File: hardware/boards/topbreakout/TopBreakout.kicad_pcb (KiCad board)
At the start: 2 copper layers, 75.6 x 73 mm, 46 parts, among them J1 WURTH_ELECTRONICS_61400413321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, J2 MOLEX_52892-3033MOLEX_52892-3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, J3 USB-A-S-X-X-VT, U1 ANALOG_DEVICES_AD7606BSTZANAL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, U3 ANALOG_DEVICES_AD5754BREZANAL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, U5 MICROCHIP_MCP1700T-2502E-TTMI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

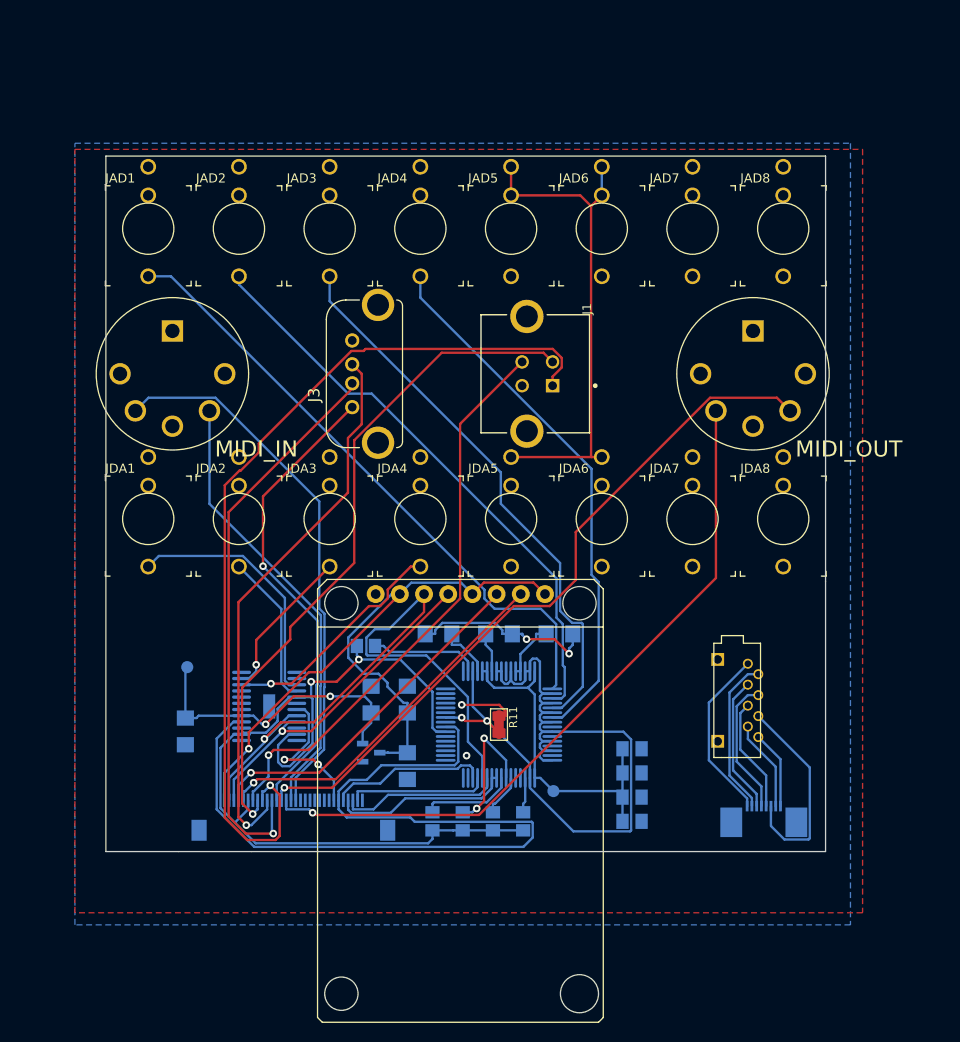
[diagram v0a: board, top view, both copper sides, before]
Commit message: cleanup
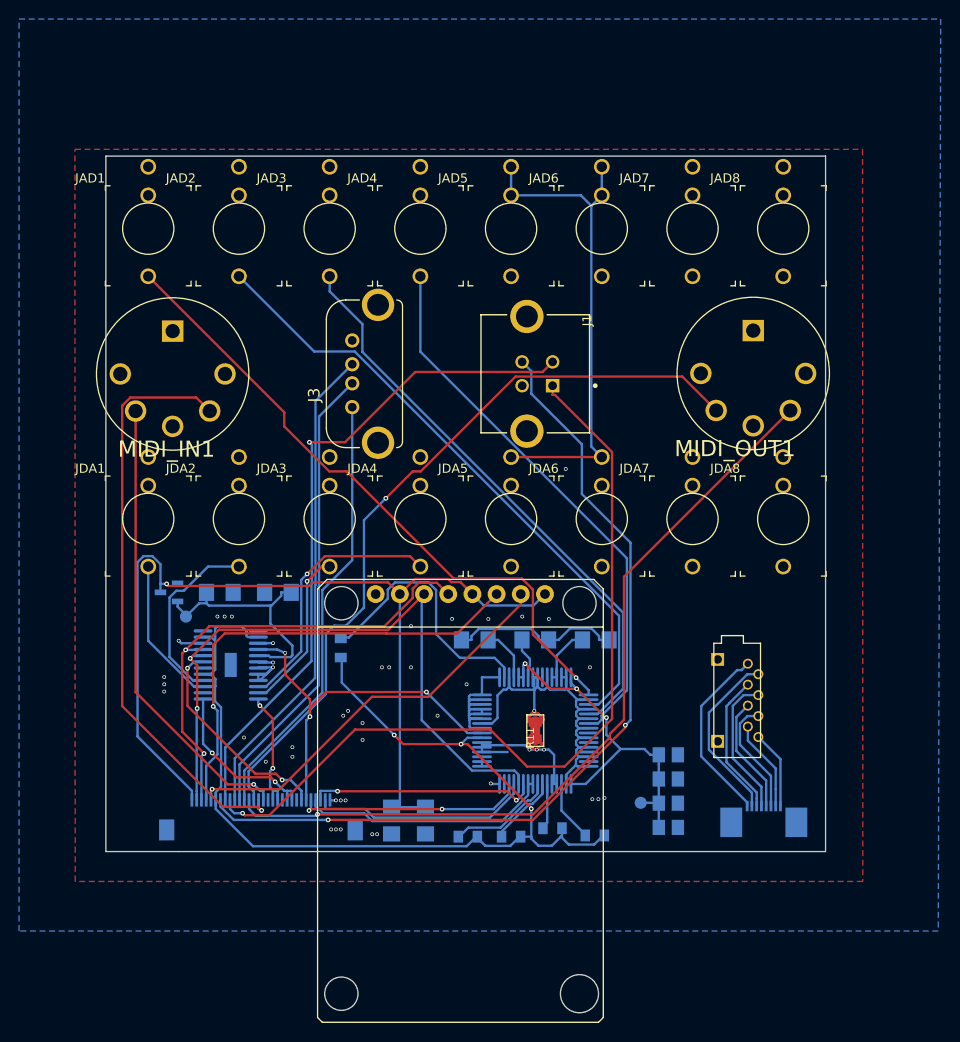
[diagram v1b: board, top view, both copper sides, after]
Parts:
- removed MIDI_IN, MIDI_OUT: OG-MIDI_MAB5SHCUI-SD-50BV, OG-MIDI_SD-50BV
- added MIDI_IN1: OG-MIDI_MAB5SHCUI-SD-50BV, topbreakout:OG-MIDI_SD-50BV, F.Cu at (117.7, 91.4)
- added MIDI_OUT1: OG-MIDI_MAB5SHCUI-SD-50BV, topbreakout:OG-MIDI_SD-50BV, F.Cu at (178.7, 91.3)
- C1, C2, C3, C4: footprint C0805K -> topbreakout:C0805K
- C10, C11, C6, C9: footprint C1206 -> topbreakout:C1206
- C5, C7, C8: footprint 1206 -> topbreakout:1206
- J1: footprint WURTH_ELECTRONICS_61400413321_0 -> topbreakout:WURTH_ELECTRONICS_61400413321_0
- J2: value MOLEX_52892-3033MOLEX_52892-3033_0_0 -> MOLEX_52892-3033; footprint MOLEX_52892-3033_0 -> topbreakout:MOLEX_52892-3033_0
- J3: footprint USB-A-S-X-X-VT -> topbreakout:USB-A-S-X-X-VT
- J4: value (none) -> ST7735_1.4; footprint ST7735 -> topbreakout:ST7735
- JAD1, JAD2, JAD3, JAD4, JAD5, JAD6, JAD7, JAD8, JDA1, JDA2, JDA3, JDA4, JDA5, JDA6, JDA7, JDA8: footprint WQP-PJ301M-12_JACK -> topbreakout:WQP-PJ301M-12_JACK
- R10, R4, R7, R8, R9: footprint R0805 -> Capacitors_SMD:C_0805
- R11: footprint R0805 -> topbreakout:R0805
- TP1, TP3: footprint PAD.03X.05 -> topbreakout:PAD.03X.05
- U$1: footprint YAMAICHI_MICROSD_VERTICAL -> topbreakout:YAMAICHI_MICROSD_VERTICAL
- U$2: footprint TE_1-1734592-8 -> topbreakout:TE_1-1734592-8
- U1: footprint ANALOG_DEVICES_AD7606BSTZ_2 -> topbreakout:ANALOG_DEVICES_AD7606BSTZ_2
- U3: footprint ANALOG_DEVICES_AD5754BREZ_2 -> topbreakout:ANALOG_DEVICES_AD5754BREZ_2
- U5: value MICROCHIP_MCP1700T-2502E-TTMICROCHIP_MCP1700T-2502E-TT_0_0 -> MCP1700T-2502E; footprint MICROCHIP_MCP1700T-2502E-TT_0 -> topbreakout:MICROCHIP_MCP1700T-2502E-TT_0
- moved U5 27.1 mm to (117.3, 114.3), turned to 180 degrees
- moved C9 15.0 mm to (122.7, 114.3), turned to 0 degrees
- moved C6 14.9 mm to (128.8, 114.3), turned to 180 degrees
- moved C10 12.8 mm to (140.7, 138.3), turned to 270 degrees
- moved TP1 9.25 mm to (166.9, 136.4)
- moved R10 7.66 mm to (162.1, 139.8), turned to 180 degrees
- moved R4 6.29 mm to (157.6, 139.1), turned to 180 degrees
- moved C11 6.02 mm to (144.3, 138.3)
- moved U3 5.94 mm to (123.8, 121.9), turned to 0 degrees
- moved R9 5.33 mm to (153.3, 140.0), turned to 0 degrees
- moved TP3 5.31 mm to (119.1, 116.8)
- moved R8 4.04 mm to (148.7, 140.0), turned to 180 degrees
- moved C2 3.86 mm to (169.8, 136.4)
- moved C1 3.86 mm to (169.8, 133.9)
- moved C3 3.86 mm to (169.8, 131.4)
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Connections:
- net AD_AGND renamed /io_breakout-ver2.1_5/AD_AGND
- net AD_BYTE_SELECT renamed /io_breakout-ver2.1_5/AD_BYTE_SELECT
- net AD_OS0 renamed /io_breakout-ver2.1_5/AD_OS0
- net AD_RANGE renamed /io_breakout-ver2.1_5/AD_RANGE
- net AD_REFCAP_A renamed /io_breakout-ver2.1_5/AD_REFCAP_A
- net AD_REFSEL renamed /io_breakout-ver2.1_5/AD_REFSEL
- net AD_REGCAP1 renamed /io_breakout-ver2.1_5/AD_REGCAP1
- net AD_REGCAP2 renamed /io_breakout-ver2.1_5/AD_REGCAP2
- net AD_STBY renamed /io_breakout-ver2.1_5/AD_STBY
- net AGND renamed /io_breakout-ver2.1_5/AGND
- net AVIN renamed /io_breakout-ver2.1_5/AVIN
- net SD_CLK renamed /io_breakout-ver2.1_3/SD_CLK
- net SD_CS renamed /io_breakout-ver2.1_3/SD_CS
- net SD_DAT1 renamed /io_breakout-ver2.1_3/SD_DAT1
- net SD_DAT2 renamed /io_breakout-ver2.1_3/SD_DAT2
- net SD_DATAIN renamed /io_breakout-ver2.1_3/SD_DATAIN
- net SD_DATAOUT renamed /io_breakout-ver2.1_3/SD_DATAOUT
- net SD_GND renamed /io_breakout-ver2.1_3/SD_GND
- net SD_VCC renamed /io_breakout-ver2.1_3/SD_VCC
- net USB_A_D+ renamed /io_breakout-ver2.1_3/USB_A_D+
- net USB_A_D- renamed /io_breakout-ver2.1_3/USB_A_D-
- net USB_A_VCC renamed /io_breakout-ver2.1_3/USB_A_VCC
- net USB_B_D+ renamed /io_breakout-ver2.1_3/USB_B_D+
- net USB_B_D- renamed /io_breakout-ver2.1_3/USB_B_D-
- net USB_B_VCC renamed /io_breakout-ver2.1_3/USB_B_VCC
- net VREF renamed /io_breakout-ver2.1_6/VREF
- J2 pad 10: (no net) -> AVSS
- J2 pad 12: (no net) -> AVDD
- J2 pad 13: (no net) -> AVDD
- J2 pad 15: MIDI_IN_PIN5 -> /io_breakout-ver2.1_3/MIDI_IN_PIN5
- J2 pad 16: MIDI_IN_PIN4 -> /io_breakout-ver2.1_3/MIDI_IN_PIN4
- J2 pad 17: MIDI_OUT_PIN5 -> /io_breakout-ver2.1_3/MIDI_OUT_PIN5
- J2 pad 18: MIDI_OUT_PIN4 -> /io_breakout-ver2.1_3/MIDI_OUT_PIN4
- J2 pad 8: N$6 -> (no net)
- J2 pad 9: (no net) -> AVSS
- JDA5 pad P$1_TIP: DA_V5 -> (no net)
- JDA6 pad P$1_TIP: DA_V6 -> (no net)
- U1 pad 42: AD_REFINOUT -> (no net)
- U1 pad 57: AD_V5 -> (no net)
- U1 pad 59: AD_V6 -> (no net)
- U1 pad 61: AD_V7 -> (no net)
- U1 pad 63: AD_V8 -> (no net)
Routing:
- net /io_breakout-ver2.1_3/MIDI_OUT_PIN4: track 0.00 -> 84.7 mm, vias 0 -> 1
- net /io_breakout-ver2.1_3/MIDI_OUT_PIN5: track 0.00 -> 80.1 mm, vias 0 -> 1
- net MIDI_OUT_PIN4: track 75.0 -> 0.00 mm, vias 1 -> 0
- net MIDI_OUT_PIN5: track 74.2 -> 0.00 mm, vias 1 -> 0
- net /io_breakout-ver2.1_3/MIDI_IN_PIN4: track 0.00 -> 62.2 mm, vias 0 -> 1
- net MIDI_IN_PIN5: track 57.2 -> 0.00 mm
- net /io_breakout-ver2.1_3/MIDI_IN_PIN5: track 0.00 -> 48.2 mm, vias 0 -> 1
- net SPI0_MISO: track 89.0 -> 41.8 mm, vias 0 -> 3
- net MIDI_IN_PIN4: track 47.0 -> 0.00 mm
- net GND: track 5.42 -> 50.9 mm, vias 2 -> 45
- net /io_breakout-ver2.1_5/AD_AGND: track 81.3 -> 48.7 mm, vias 2 -> 1
- net /io_breakout-ver2.1_3/USB_B_D+: track 60.0 -> 91.1 mm, vias 1 -> 2
- net VIN: track 73.3 -> 102.7 mm
- net AVSS: track 0.00 -> 17.9 mm, vias 0 -> 2
- net /io_breakout-ver2.1_5/AD_REFSEL: track 11.5 -> 27.4 mm
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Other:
- rule trace_min: 0.2 -> 0.12
- rule via_min_drill: 0.3 -> 0.25
